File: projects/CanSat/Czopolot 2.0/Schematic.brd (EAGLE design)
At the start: 57 x 32.8 mm, 96 parts, among them X1 FH12-24S-0.5SH

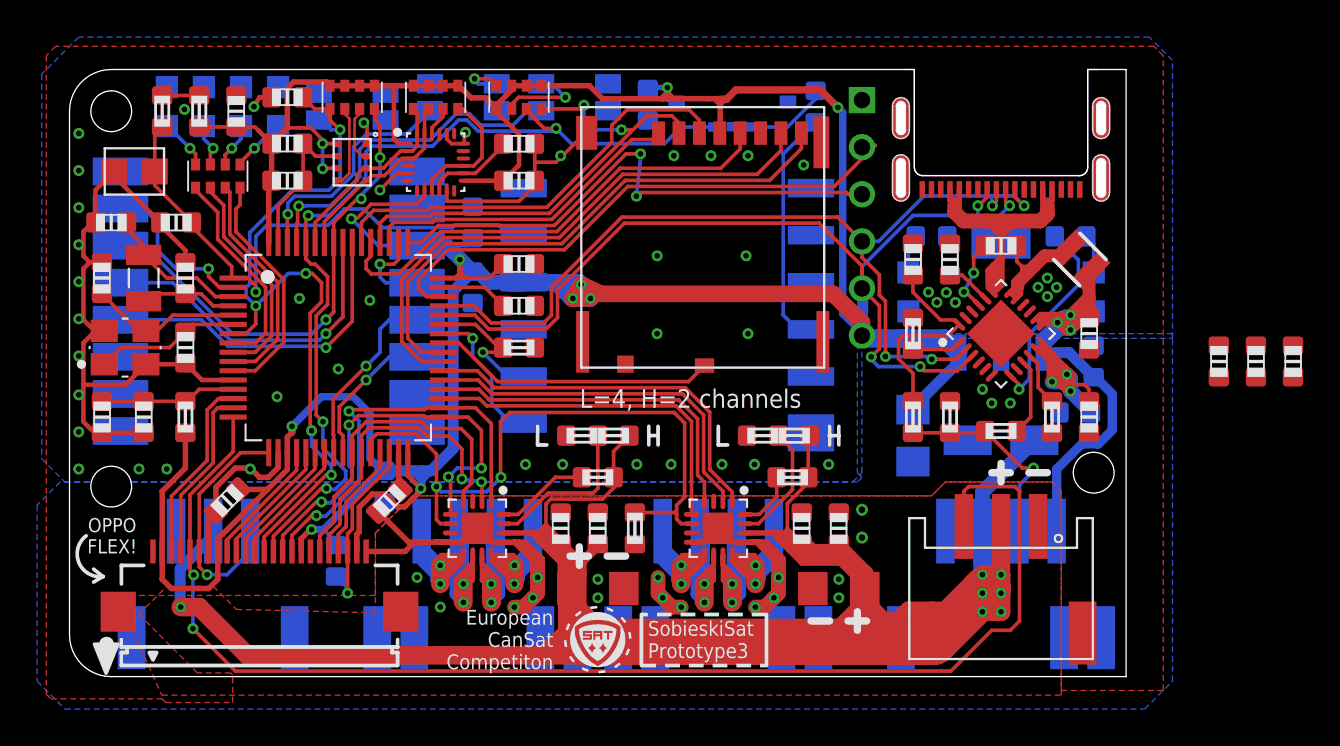
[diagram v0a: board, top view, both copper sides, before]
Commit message: Before ordering
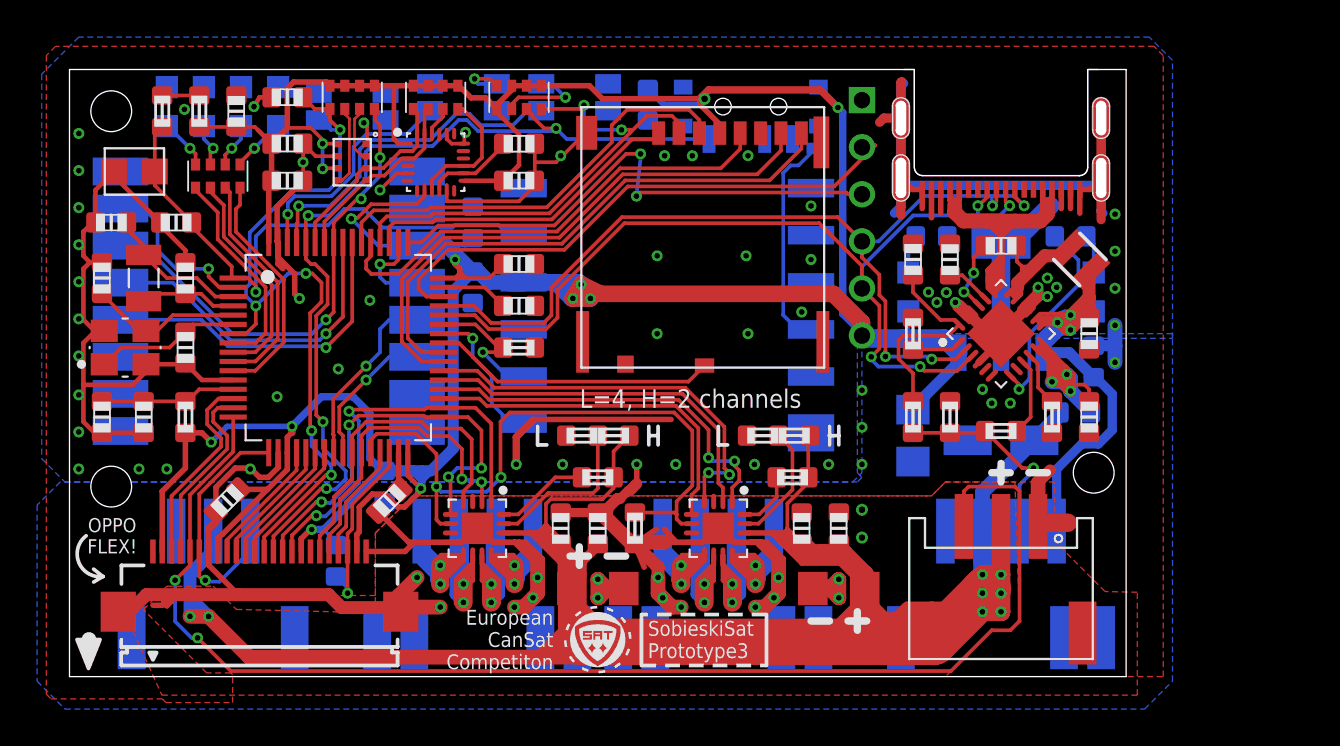
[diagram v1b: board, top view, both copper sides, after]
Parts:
- removed C10: 10n, Unified:C0603
- removed C2: 10u, Unified:C0603
- removed C81: 100n, Unified:C0603
- removed R10: 0R, Unified:R0603
- removed U$23: LOGOSQSM, SobieskiSat2:LOGOSQSM
- BTN_DFU: value SLIDE-SWITCH -> SLIDE-SWITCH2; device SobieskiSat2:SLIDE-SWITCH -> SobieskiSat2:SLIDE-SWITCH-2
- U$22: value LOGORICK -> PADSMALL; device SobieskiSat2:RICK -> Unified:SMALL_PAD
- moved U$22 13.5 mm to (40.2, 28.5), turned to 270 degrees
- moved BTN_DFU 1.03 mm to (36.8, 30.8)
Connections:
- removed net N$25: BTN_DFU.P$1, R10.1
- net BAT: no longer C10.1
- net GND: no longer C10.2, C2.2, C81.2
- net GPS_RST: now also U$22.P$1; no longer R10.2
- net PWM_4: now also U$11.4; no longer U$11.1
- net P_EN_4: now also U$11.1; no longer U$11.4
- net VCC: no longer C81.1
- net VSYS: no longer C2.1
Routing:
- net GND: track 110.3 -> 254.9 mm, vias 66 -> 76
- net N$25: track 4.56 -> 0.00 mm
- net BAT: track 155.0 -> 159.5 mm, vias 7 -> 8
- net VCC: track 209.5 -> 207.0 mm, vias 12 -> 13
- net P_EN_4: track 19.0 -> 20.6 mm, vias 0 -> 2
- net PWM_4: track 20.6 -> 21.9 mm, vias 0 -> 2
- net GPS_RST: track 13.0 -> 11.8 mm
- net UART2_TX: track 71.2 -> 72.2 mm
- net DFU: track 49.9 -> 49.2 mm
- net GPS_TX: track 8.44 -> 7.69 mm
- net UART4_TX: track 10.1 -> 10.7 mm
- net UART4_RX: track 9.41 -> 10.0 mm
- net UART2_RX: track 13.1 -> 13.7 mm
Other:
- outline, holes or cut-outs redrawn
- board text removed: "-------- SobieskiSat Prototype3 -------- European CanSat Competiton -------- Poland 2020 --------"
- board text removed: "RST"
